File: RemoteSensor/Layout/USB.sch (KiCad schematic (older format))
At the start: 17 parts, among them Q4 MMBT2222A-TP, Q5 MMBT2222A-TP, U10 FT231XS

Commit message: Update PCB layout
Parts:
- removed D3, D4: LED, LED_SMD:LED_0603_1608Metric_Pad1.05x0.95mm_HandSolder, symbol Device:LED
- removed R27, R28: 100, Resistor_SMD:R_0603_1608Metric_Pad1.05x0.95mm_HandSolder, symbol Device:R_US
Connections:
- wire segments 52 -> 44
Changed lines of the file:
@@
 Connection ~ 5050 3800
-Wire Wire Line
-	4950 3600 5200 3600
 Wire Wire Line
 	4550 3500 5200 3500
@@
 	1    0    0    -1
 $EndComp
-$Comp
-L Device:LED D3
-U 1 1 5EF0F904
-P 6750 4800
-F 0 "D3" V 6697 4878 50  0000 L CNN
-F 1 "LED" V 6788 4878 50  0000 L CNN
-F 2 "LED_SMD:LED_0603_1608Metric_Pad1.05x0.95mm_HandSolder" H 6750 4800 50  0001 C CNN
-F 3 "~" H 6750 4800 50  0001 C CNN
-	1    6750 4800
-	0    1    1    0
-$EndComp
-$Comp
-L Device:LED D4
-U 1 1 5EF109F5
-P 7150 4800
-F 0 "D4" V 7097 4878 50  0000 L CNN
-F 1 "LED" V 7188 4878 50  0000 L CNN
-F 2 "LED_SMD:LED_0603_1608Metric_Pad1.05x0.95mm_HandSolder" H 7150 4800 50  0001 C CNN
-F 3 "~" H 7150 4800 50  0001 C CNN
-	1    7150 4800
-	0    1    1    0
-$EndComp
-Wire Wire Line
-	6600 4300 6750 4300
-Wire Wire Line
-	6750 4300 6750 4650
-Wire Wire Line
-	6600 4200 7150 4200
-Wire Wire Line
-	7150 4200 7150 4650
-$Comp
-L Device:R_US R27
-U 1 1 5EF1163C
-P 6750 5100
-F 0 "R27" H 6818 5146 50  0000 L CNN
-F 1 "100" H 6818 5055 50  0000 L CNN
-F 2 "Resistor_SMD:R_0603_1608Metric_Pad1.05x0.95mm_HandSolder" V 6790 5090 50  0001 C CNN
-F 3 "~" H 6750 5100 50  0001 C CNN
-	1    6750 5100
-	1    0    0    -1
-$EndComp
-$Comp
-L Device:R_US R28
-U 1 1 5EF11D39
-P 7150 5100
-F 0 "R28" H 7218 5146 50  0000 L CNN
-F 1 "100" H 7218 5055 50  0000 L CNN
-F 2 "Resistor_SMD:R_0603_1608Metric_Pad1.05x0.95mm_HandSolder" V 7190 5090 50  0001 C CNN
-F 3 "~" H 7150 5100 50  0001 C CNN
-	1    7150 5100
-	1    0    0    -1
-$EndComp
-Wire Wire Line
-	6750 5250 6750 5400
-Wire Wire Line
-	6750 5400 7150 5400
-Wire Wire Line
-	7150 5400 7150 5250
-Wire Wire Line
-	7150 5400 7900 5400
-Connection ~ 7150 5400
-Text Label 7900 5400 2    50   ~ 0
-VCCIO
 $Comp
 L Device:C C9
@@
 Text Label 8600 3400 2    50   ~ 0
 RTS
+Wire Wire Line
+	4650 4300 4650 4850
+Wire Wire Line
+	4650 4850 5800 4850
+Wire Wire Line
+	6000 4850 6000 4700
+Wire Wire Line
+	5800 4700 5800 4850
+Connection ~ 5800 4850
+Wire Wire Line
+	5800 4850 6000 4850
+$Comp
+L RemoteSensor-rescue:GND-SparkFun-PowerSymbols #GND0113
+U 1 1 5EF4CBA7
+P 6000 4850
+F 0 "#GND0113" H 6050 4800 45  0001 L BNN
+F 1 "GND" H 6000 4680 45  0000 C CNN
+F 2 "" H 6000 4750 60  0001 C CNN
+F 3 "" H 6000 4750 60  0001 C CNN
+	1    6000 4850
+	1    0    0    -1
+$EndComp
+Connection ~ 6000 4850
+Text Label 8600 3600 2    50   ~ 0
+DTR
+Wire Wire Line
+	4950 3600 5200 3600
 $Comp
 L Interface_USB:FT231XS U10
@@
 	1    0    0    -1
 $EndComp
-Wire Wire Line
-	4650 4300 4650 4850
-Wire Wire Line
-	4650 4850 5800 4850
-Wire Wire Line
-	6000 4850 6000 4700
-Wire Wire Line
-	5800 4700 5800 4850
-Connection ~ 5800 4850
-Wire Wire Line
-	5800 4850 6000 4850
-$Comp
-L RemoteSensor-rescue:GND-SparkFun-PowerSymbols #GND0113
-U 1 1 5EF4CBA7
-P 6000 4850
-F 0 "#GND0113" H 6050 4800 45  0001 L BNN
-F 1 "GND" H 6000 4680 45  0000 C CNN
-F 2 "" H 6000 4750 60  0001 C CNN
-F 3 "" H 6000 4750 60  0001 C CNN
-	1    6000 4850
-	1    0    0    -1
-$EndComp
-Connection ~ 6000 4850
-Text Label 8600 3600 2    50   ~ 0
-DTR
 $EndSCHEMATC

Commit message: Change what pins are used for i2c
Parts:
- C10, C8, C9: symbol Device:C -> RemoteSensor-rescue:C-Device
- FB1: symbol Device:Ferrite_Bead -> RemoteSensor-rescue:Ferrite_Bead-Device
- JP1, JP2: symbol Jumper:Jumper_2_Open -> RemoteSensor-rescue:Jumper_2_Open-Jumper
- R23, R24, R25, R26: symbol Device:R_US -> RemoteSensor-rescue:R_US-Device
- U10: symbol Interface_USB:FT231XS -> RemoteSensor-rescue:FT231XS-Interface_USB
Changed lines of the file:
@@
 $EndDescr
 $Comp
-L Device:Ferrite_Bead FB1
+L RemoteSensor-rescue:Ferrite_Bead-Device FB1
 U 1 1 5EF07BAD
 P 5800 2350
@@
 $EndComp
 $Comp
-L Device:R_US R25
+L RemoteSensor-rescue:R_US-Device R25
 U 1 1 5EF0826F
 P 4400 3500
@@
 $EndComp
 $Comp
-L Device:R_US R26
+L RemoteSensor-rescue:R_US-Device R26
 U 1 1 5EF088E2
 P 4800 3600
@@
 	5050 3800 5200 3800
 $Comp
-L Device:C C10
+L RemoteSensor-rescue:C-Device C10
 U 1 1 5EF0B19A
 P 5050 4150
@@
 Connection ~ 5050 3200
 $Comp
-L Jumper:Jumper_2_Open JP1
+L RemoteSensor-rescue:Jumper_2_Open-Jumper JP1
 U 1 1 5EF0D6FF
 P 7200 3600
@@
 $EndComp
 $Comp
-L Jumper:Jumper_2_Open JP2
+L RemoteSensor-rescue:Jumper_2_Open-Jumper JP2
 U 1 1 5EF0E1DD
 P 7850 3400
@@
 $EndComp
 $Comp
-L Device:C C9
+L RemoteSensor-rescue:C-Device C9
 U 1 1 5EF16A27
 P 4650 4150
@@
 $EndComp
 $Comp
-L Device:C C8
+L RemoteSensor-rescue:C-Device C8
 U 1 1 5EF171E4
 P 4250 4150
@@
 $EndComp
 $Comp
-L Device:R_US R23
+L RemoteSensor-rescue:R_US-Device R23
 U 1 1 5EF30FEC
 P 2150 5500
@@
 $EndComp
 $Comp
-L Device:R_US R24
+L RemoteSensor-rescue:R_US-Device R24
 U 1 1 5EF32BAD
 P 2150 6350
@@
 	4950 3600 5200 3600
 $Comp
-L Interface_USB:FT231XS U10
+L RemoteSensor-rescue:FT231XS-Interface_USB U10
 U 1 1 5EF43B07
 P 5900 3800

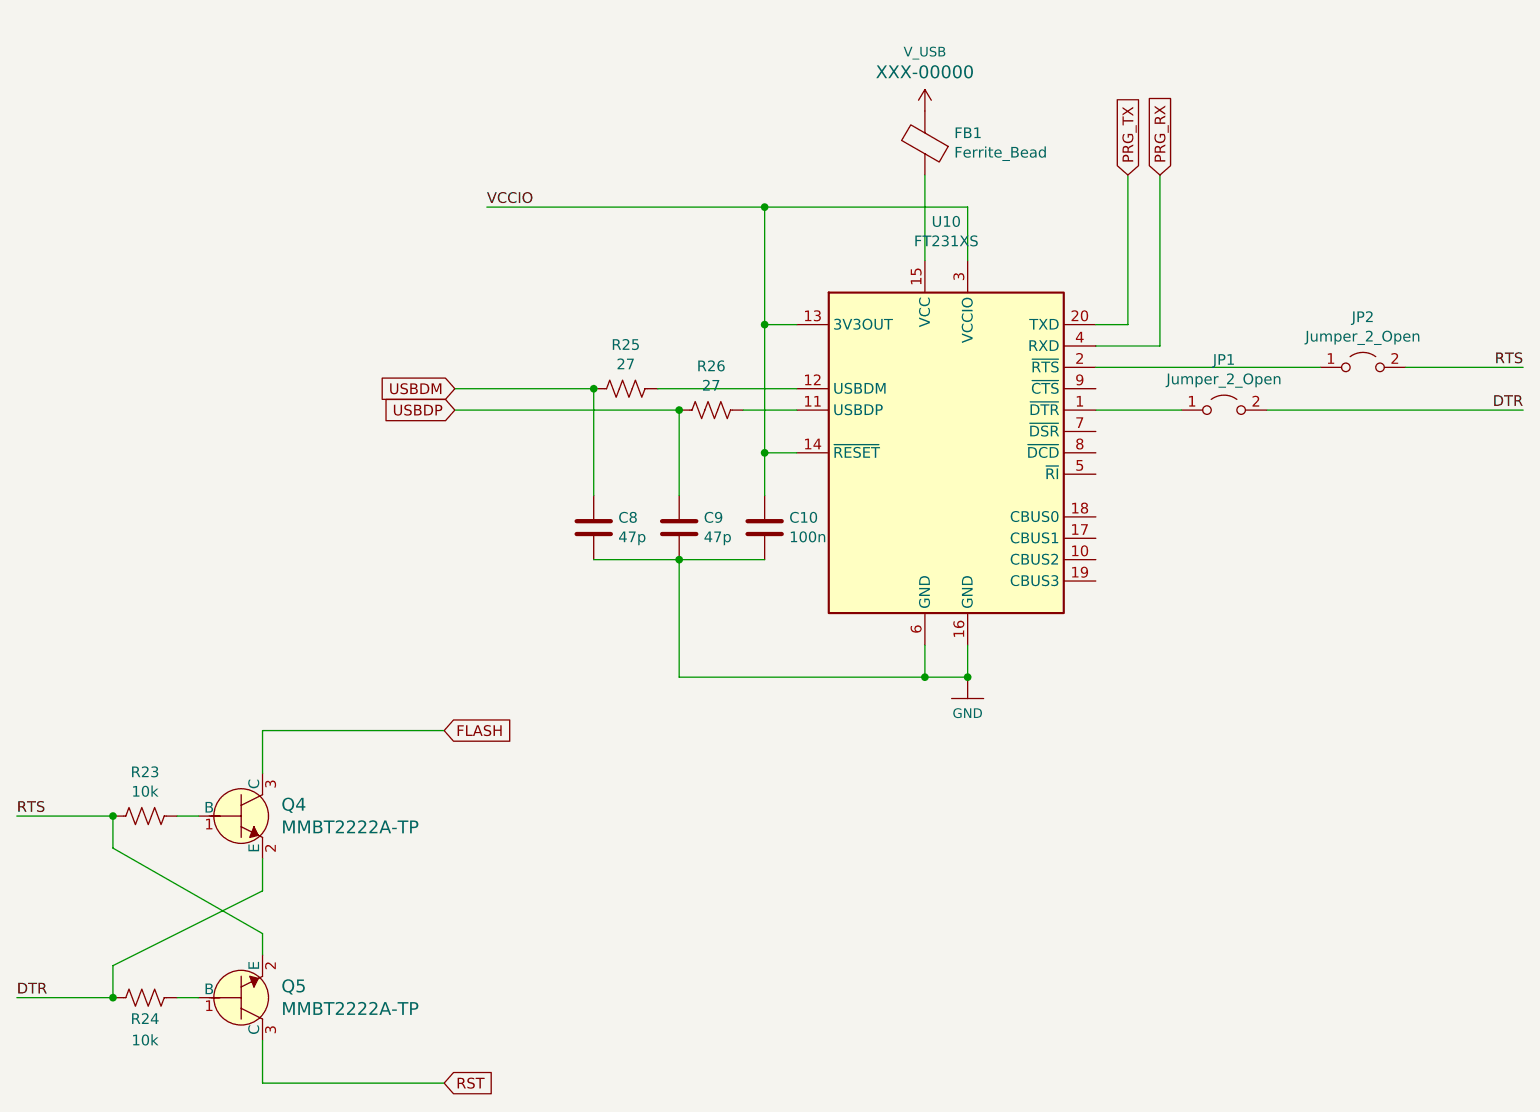
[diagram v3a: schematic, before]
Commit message: Another layout
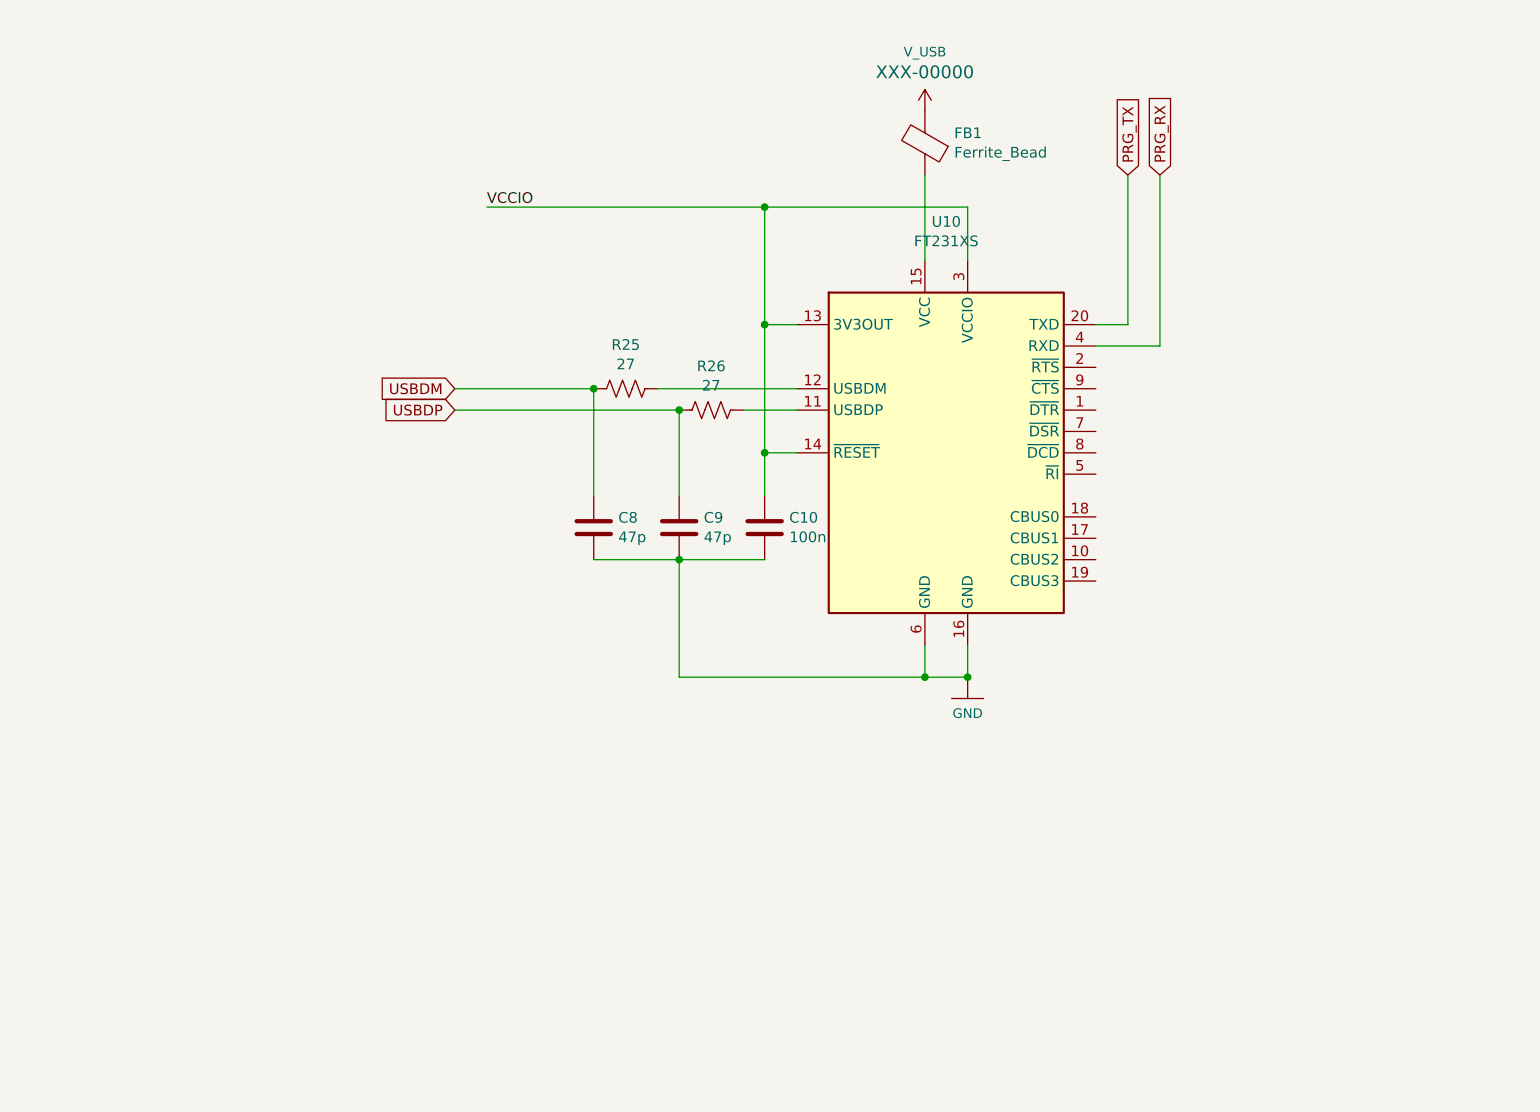
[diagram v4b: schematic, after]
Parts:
- removed JP1, JP2: Jumper_2_Open, Jumper:SolderJumper-2_P1.3mm_Open_Pad1.0x1.5mm, symbol RemoteSensor-rescue:Jumper_2_Open-Jumper
- removed Q4, Q5: MMBT2222A-TP, digikey-footprints:SOT-23-3, symbol RemoteSensor-rescue:MMBT2222A-TP-dk_Transistors-Bipolar-BJT-Single
- removed R23, R24: 10k, Resistor_SMD:R_0603_1608Metric_Pad1.05x0.95mm_HandSolder, symbol RemoteSensor-rescue:R_US-Device
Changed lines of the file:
@@
 Connection ~ 5050 3200
-$Comp
-L RemoteSensor-rescue:Jumper_2_Open-Jumper JP1
-U 1 1 5EF0D6FF
-P 7200 3600
-F 0 "JP1" H 7200 3835 50  0000 C CNN
-F 1 "Jumper_2_Open" H 7200 3744 50  0000 C CNN
-F 2 "Jumper:SolderJumper-2_P1.3mm_Open_Pad1.0x1.5mm" H 7200 3600 50  0001 C CNN
-F 3 "~" H 7200 3600 50  0001 C CNN
-	1    7200 3600
-	1    0    0    -1
-$EndComp
-$Comp
-L RemoteSensor-rescue:Jumper_2_Open-Jumper JP2
-U 1 1 5EF0E1DD
-P 7850 3400
-F 0 "JP2" H 7850 3635 50  0000 C CNN
-F 1 "Jumper_2_Open" H 7850 3544 50  0000 C CNN
-F 2 "Jumper:SolderJumper-2_P1.3mm_Open_Pad1.0x1.5mm" H 7850 3400 50  0001 C CNN
-F 3 "~" H 7850 3400 50  0001 C CNN
-	1    7850 3400
-	1    0    0    -1
-$EndComp
-Wire Wire Line
-	7650 3400 6600 3400
-Wire Wire Line
-	6600 3600 7000 3600
 $Comp
 L RemoteSensor-rescue:V_USB-SparkFun-PowerSymbols #SUPPLY0122
@@
 PRG_TX
 Wire Wire Line
-	7400 3600 8600 3600
-Wire Wire Line
-	8050 3400 8600 3400
-Text Label 8600 3400 2    50   ~ 0
-RTS
-Wire Wire Line
 	4650 4300 4650 4850
 Wire Wire Line
@@
 $EndComp
 Connection ~ 6000 4850
-Text Label 8600 3600 2    50   ~ 0
-DTR
 Wire Wire Line
 	4950 3600 5200 3600
@@
 	1    0    0    -1
 $EndComp
-Text GLabel 3550 6750 2    50   Input ~ 0
-RST
-Text GLabel 3550 5100 2    50   Input ~ 0
-FLASH
-Text Label 1550 6350 0    50   ~ 0
-DTR
-Text Label 1550 5500 0    50   ~ 0
-RTS
-Wire Wire Line
-	2700 6750 3550 6750
-Wire Wire Line
-	2700 6550 2700 6750
-Wire Wire Line
-	2700 5100 3550 5100
-Wire Wire Line
-	2700 5300 2700 5100
-Wire Wire Line
-	2000 5500 1550 5500
-Wire Wire Line
-	2000 6350 1550 6350
-Wire Wire Line
-	2000 6200 2000 6350
-Wire Wire Line
-	2700 5850 2000 6200
-Wire Wire Line
-	2700 5700 2700 5850
-Wire Wire Line
-	2000 5650 2000 5500
-Wire Wire Line
-	2700 6050 2000 5650
-Wire Wire Line
-	2700 6150 2700 6050
-Wire Wire Line
-	2300 5500 2400 5500
-Wire Wire Line
-	2300 6350 2400 6350
-Connection ~ 2000 6350
-$Comp
-L RemoteSensor-rescue:R_US-Device R24
-U 1 1 5EF32BAD
-P 2150 6350
-F 0 "R24" V 2250 6350 50  0000 C CNN
-F 1 "10k" V 2350 6350 50  0000 C CNN
-F 2 "Resistor_SMD:R_0603_1608Metric_Pad1.05x0.95mm_HandSolder" V 2190 6340 50  0001 C CNN
-F 3 "~" H 2150 6350 50  0001 C CNN
-	1    2150 6350
-	0    1    1    0
-$EndComp
-Connection ~ 2000 5500
-$Comp
-L RemoteSensor-rescue:R_US-Device R23
-U 1 1 5EF30FEC
-P 2150 5500
-F 0 "R23" V 1945 5500 50  0000 C CNN
-F 1 "10k" V 2036 5500 50  0000 C CNN
-F 2 "Resistor_SMD:R_0603_1608Metric_Pad1.05x0.95mm_HandSolder" V 2190 5490 50  0001 C CNN
-F 3 "~" H 2150 5500 50  0001 C CNN
-	1    2150 5500
-	0    1    1    0
-$EndComp
-$Comp
-L RemoteSensor-rescue:MMBT2222A-TP-dk_Transistors-Bipolar-BJT-Single Q5
-U 1 1 5EF2EBF2
-P 2600 6350
-F 0 "Q5" H 2788 6297 60  0000 L CNN
-F 1 "MMBT2222A-TP" H 2788 6403 60  0000 L CNN
-F 2 "digikey-footprints:SOT-23-3" H 2800 6550 60  0001 L CNN
-F 3 "https://www.mccsemi.com/pdf/Products/MMBT2222A(SOT-23).pdf" H 2800 6650 60  0001 L CNN
-F 4 "MMBT2222ATPMSCT-ND" H 2800 6750 60  0001 L CNN "Digi-Key_PN"
-F 5 "MMBT2222A-TP" H 2800 6850 60  0001 L CNN "MPN"
-F 6 "Discrete Semiconductor Products" H 2800 6950 60  0001 L CNN "Category"
-F 7 "Transistors - Bipolar (BJT) - Single" H 2800 7050 60  0001 L CNN "Family"
-F 8 "https://www.mccsemi.com/pdf/Products/MMBT2222A(SOT-23).pdf" H 2800 7150 60  0001 L CNN "DK_Datasheet_Link"
-F 9 "/product-detail/en/micro-commercial-co/MMBT2222A-TP/MMBT2222ATPMSCT-ND/717394" H 2800 7250 60  0001 L CNN "DK_Detail_Page"
-F 10 "TRANS NPN 40V 0.6A SOT23" H 2800 7350 60  0001 L CNN "Description"
-F 11 "Micro Commercial Co" H 2800 7450 60  0001 L CNN "Manufacturer"
-F 12 "Active" H 2800 7550 60  0001 L CNN "Status"
-	1    2600 6350
-	1    0    0    1
-$EndComp
-$Comp
-L RemoteSensor-rescue:MMBT2222A-TP-dk_Transistors-Bipolar-BJT-Single Q4
-U 1 1 5EF2CE7F
-P 2600 5500
-F 0 "Q4" H 2788 5553 60  0000 L CNN
-F 1 "MMBT2222A-TP" H 2788 5447 60  0000 L CNN
-F 2 "digikey-footprints:SOT-23-3" H 2800 5700 60  0001 L CNN
-F 3 "https://www.mccsemi.com/pdf/Products/MMBT2222A(SOT-23).pdf" H 2800 5800 60  0001 L CNN
-F 4 "MMBT2222ATPMSCT-ND" H 2800 5900 60  0001 L CNN "Digi-Key_PN"
-F 5 "MMBT2222A-TP" H 2800 6000 60  0001 L CNN "MPN"
-F 6 "Discrete Semiconductor Products" H 2800 6100 60  0001 L CNN "Category"
-F 7 "Transistors - Bipolar (BJT) - Single" H 2800 6200 60  0001 L CNN "Family"
-F 8 "https://www.mccsemi.com/pdf/Products/MMBT2222A(SOT-23).pdf" H 2800 6300 60  0001 L CNN "DK_Datasheet_Link"
-F 9 "/product-detail/en/micro-commercial-co/MMBT2222A-TP/MMBT2222ATPMSCT-ND/717394" H 2800 6400 60  0001 L CNN "DK_Detail_Page"
-F 10 "TRANS NPN 40V 0.6A SOT23" H 2800 6500 60  0001 L CNN "Description"
-F 11 "Micro Commercial Co" H 2800 6600 60  0001 L CNN "Manufacturer"
-F 12 "Active" H 2800 6700 60  0001 L CNN "Status"
-	1    2600 5500
-	1    0    0    -1
-$EndComp
